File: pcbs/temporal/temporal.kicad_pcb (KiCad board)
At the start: 2 copper layers, 147.4 x 108 mm, 60 parts

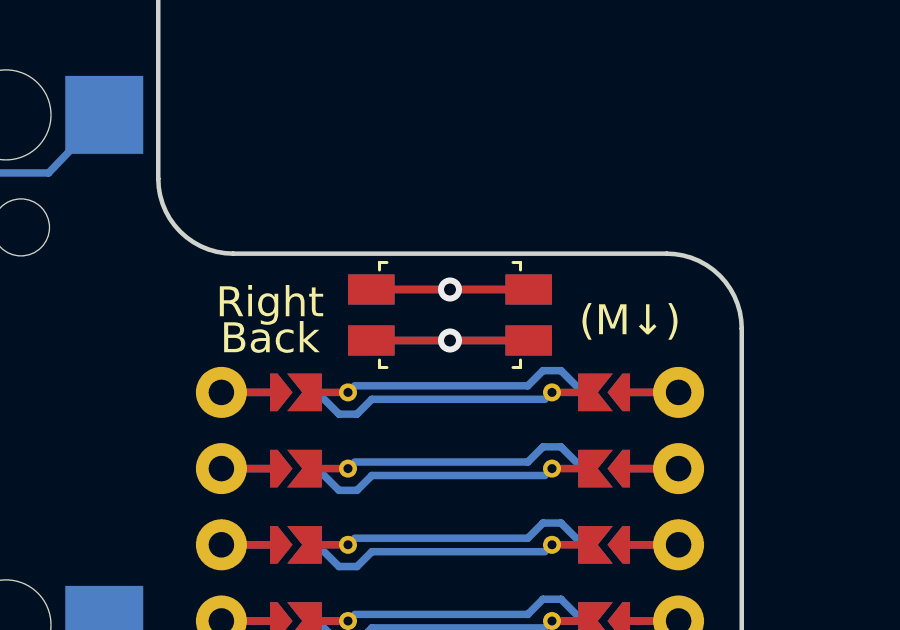
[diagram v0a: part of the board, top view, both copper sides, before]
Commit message: update gen files
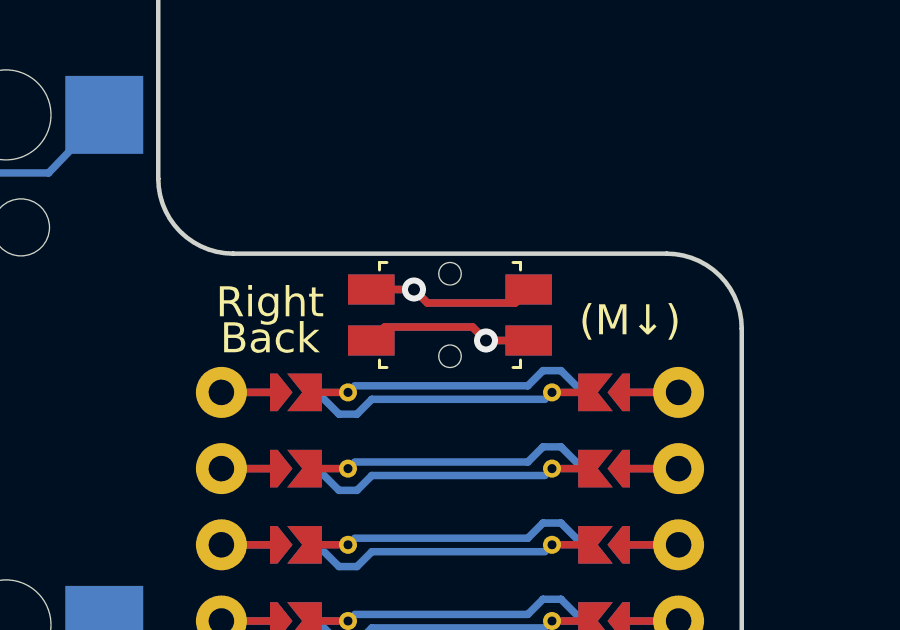
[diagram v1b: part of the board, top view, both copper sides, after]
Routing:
- net GND: track 17.9 -> 18.6 mm
- net RST: track 10.5 -> 11.2 mm
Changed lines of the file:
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@@
   (title_block
     (title "temporal")
-    (date "2025-11-24")
+    (date "2025-11-25")
     (rev "1")
     (company "Curtis Bollinger")
@@
     (fp_line (start 1.3 -2.75) (end 1.3 -1.75) (stroke (width 0.1) (type solid)) (layer "Dwgs.User"))
     (fp_line (start 2.35 -1.75) (end 2.35 1.75) (stroke (width 0.1) (type solid)) (layer "Dwgs.User"))
+    (pad "" np_thru_hole circle (at 0 -1.375 180) (size 0.75 0.75) (drill 0.75) (layers "*.Cu" "*.Mask"))
+    (pad "" np_thru_hole circle (at 0 1.375 180) (size 0.75 0.75) (drill 0.75) (layers "*.Cu" "*.Mask"))
     (pad "1" smd rect (at 2.625 -0.85 180) (size 1.55 1) (layers "F.Cu" "F.Paste" "F.Mask") (net 3 "GND"))
     (pad "2" smd rect (at 2.625 0.85 180) (size 1.55 1) (layers "F.Cu" "F.Paste" "F.Mask") (net 39 "RST"))
@@
     (fp_line (start 2.35 1.5) (end 2.35 1.75) (stroke (width 0.1) (type solid)) (layer "B.SilkS"))
   )
-    (via (at 156.2228753 42.29143700000001) (size 0.8) (drill 0.4) (layers "F.Cu" "B.Cu") (net 3))
-    (segment (start 153.5978753 42.29143700000001) (end 156.2228753 42.29143700000001) (width 0.25) (layer "F.Cu") (net 3))
-    (segment (start 158.8478753 42.29143700000001) (end 156.2228753 42.29143700000001) (width 0.25) (layer "F.Cu") (net 3))
-    (segment (start 153.5978753 42.29143700000001) (end 156.2228753 42.29143700000001) (width 0.25) (layer "B.Cu") (net 3))
-    (segment (start 158.8478753 42.29143700000001) (end 156.2228753 42.29143700000001) (width 0.25) (layer "B.Cu") (net 3))
-    (via (at 156.2228753 43.99143700000001) (size 0.8) (drill 0.4) (layers "F.Cu" "B.Cu") (net 39))
-    (segment (start 153.5978753 43.99143700000001) (end 156.2228753 43.99143700000001) (width 0.25) (layer "F.Cu") (net 39))
-    (segment (start 158.8478753 43.99143700000001) (end 156.2228753 43.99143700000001) (width 0.25) (layer "F.Cu") (net 39))
-    (segment (start 153.5978753 43.99143700000001) (end 156.2228753 43.99143700000001) (width 0.25) (layer "B.Cu") (net 39))
-    (segment (start 158.8478753 43.99143700000001) (end 156.2228753 43.99143700000001) (width 0.25) (layer "B.Cu") (net 39))
+    (via (at 155.0228753 42.29143700000001) (size 0.8) (drill 0.4) (layers "F.Cu" "B.Cu") (net 3))
+    (segment (start 153.5978753 42.29143700000001) (end 155.0228753 42.29143700000001) (width 0.25) (layer "F.Cu") (net 3))
+    (segment (start 158.8478753 42.29143700000001) (end 158.3978753 42.74143700000001) (width 0.25) (layer "F.Cu") (net 3))
+    (segment (start 158.3978753 42.74143700000001) (end 155.4728753 42.74143700000001) (width 0.25) (layer "F.Cu") (net 3))
+    (segment (start 155.4728753 42.74143700000001) (end 155.0228753 42.29143700000001) (width 0.25) (layer "F.Cu") (net 3))
+    (segment (start 153.5978753 42.29143700000001) (end 155.0228753 42.29143700000001) (width 0.25) (layer "B.Cu") (net 3))
+    (segment (start 158.8478753 42.29143700000001) (end 158.3978753 42.74143700000001) (width 0.25) (layer "B.Cu") (net 3))
+    (segment (start 158.3978753 42.74143700000001) (end 155.4728753 42.74143700000001) (width 0.25) (layer "B.Cu") (net 3))
+    (segment (start 155.4728753 42.74143700000001) (end 155.0228753 42.29143700000001) (width 0.25) (layer "B.Cu") (net 3))
+    (via (at 157.4228753 43.99143700000001) (size 0.8) (drill 0.4) (layers "F.Cu" "B.Cu") (net 39))
+    (segment (start 158.8478753 43.99143700000001) (end 157.4228753 43.99143700000001) (width 0.25) (layer "F.Cu") (net 39))
+    (segment (start 153.5978753 43.99143700000001) (end 154.0478753 43.54143700000001) (width 0.25) (layer "F.Cu") (net 39))
+    (segment (start 154.0478753 43.54143700000001) (end 156.9728753 43.54143700000001) (width 0.25) (layer "F.Cu") (net 39))
+    (segment (start 156.9728753 43.54143700000001) (end 157.4228753 43.99143700000001) (width 0.25) (layer "F.Cu") (net 39))
+    (segment (start 158.8478753 43.99143700000001) (end 157.4228753 43.99143700000001) (width 0.25) (layer "B.Cu") (net 39))
+    (segment (start 153.5978753 43.99143700000001) (end 154.0478753 43.54143700000001) (width 0.25) (layer "B.Cu") (net 39))
+    (segment (start 154.0478753 43.54143700000001) (end 156.9728753 43.54143700000001) (width 0.25) (layer "B.Cu") (net 39))
+    (segment (start 156.9728753 43.54143700000001) (end 157.4228753 43.99143700000001) (width 0.25) (layer "B.Cu") (net 39))
   (footprint "ceoloide:power_switch_smd_side"
     (layer "F.Cu")
